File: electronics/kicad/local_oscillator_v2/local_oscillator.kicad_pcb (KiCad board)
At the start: 2 copper layers, 12 parts, among them P1 TestPoint:TestPoint_Pad_1.5x1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, P2 TestPoint:TestPoint_Pad_1.5x1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, P3 TestPoint:TestPoint_Pad_1.5x1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, U1 CE3520K3

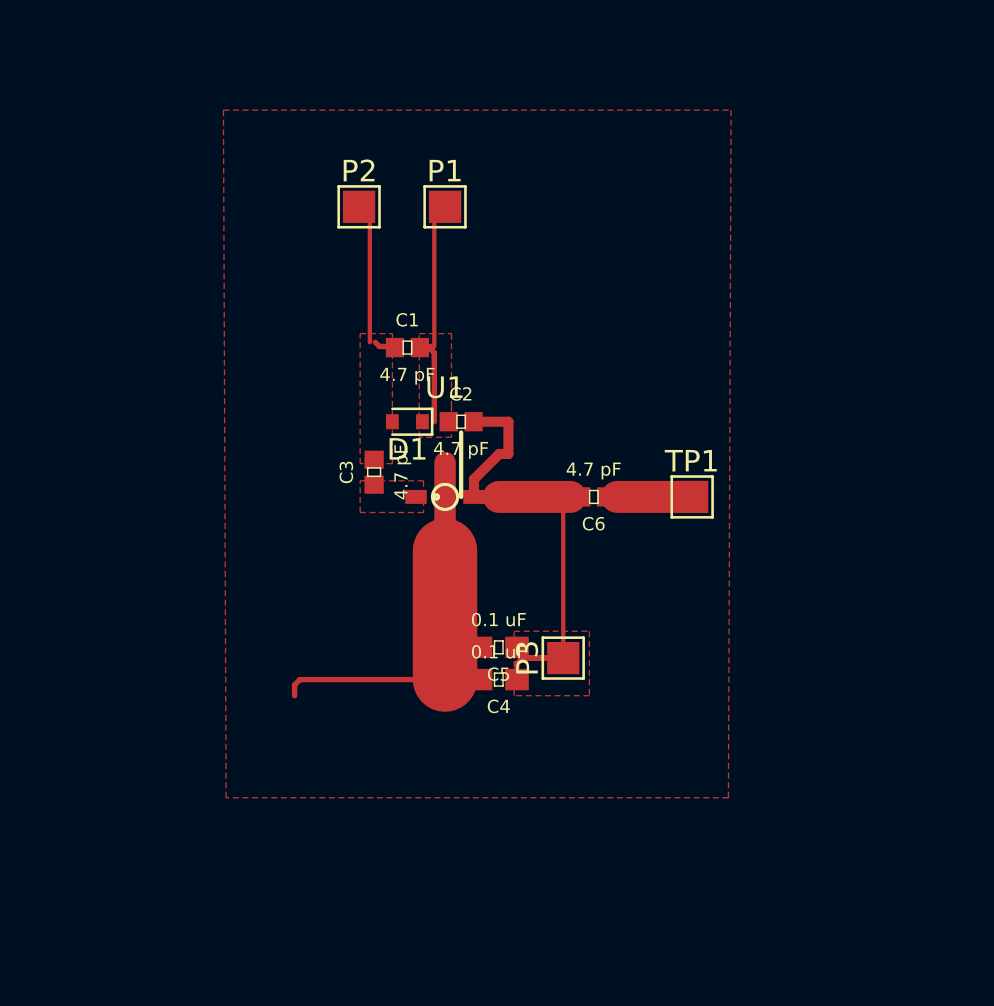
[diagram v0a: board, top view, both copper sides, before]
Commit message: Notch filter
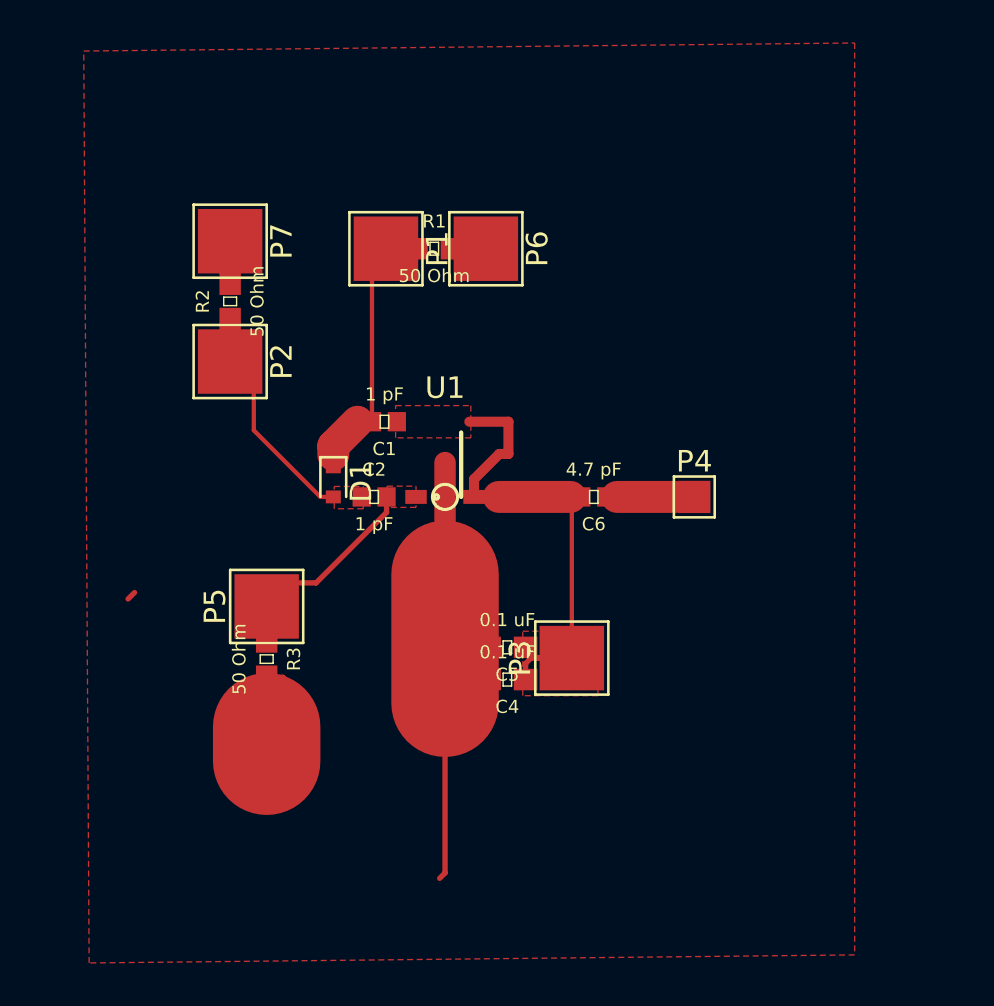
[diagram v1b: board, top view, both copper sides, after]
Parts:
- removed C3: 4.7 pF, 0402
- removed TP1: SMA, TestPoint:TestPoint_Pad_1.5x1.5mm
- added P4: TestPoint:TestPoint_Pad_1.5x1.5mm, TestPoint:TestPoint_Pad_1.5x1.5mm, F.Cu at (72.6, 44.0)
- added P5: TestPoint:TestPoint_Pad_1.5x1.5mm, TestPoint:TestPoint_Pad_3.0x3.0mm, F.Cu at (52.7, 49.1)
- added P6: TestPoint:TestPoint_Pad_1.5x1.5mm, TestPoint:TestPoint_Pad_3.0x3.0mm, F.Cu at (62.9, 32.5)
- added P7: TestPoint:TestPoint_Pad_1.5x1.5mm, TestPoint:TestPoint_Pad_3.0x3.0mm, F.Cu at (51.0, 32.1)
- added R1: 50 Ohm, Capacitors:0603, F.Cu at (60.5, 32.5)
- added R2: 50 Ohm, Capacitors:0603, F.Cu at (51.0, 34.9)
- added R3: 50 Ohm, Capacitors:0603, F.Cu at (52.7, 51.5)
- C1: value 4.7 pF -> 1 pF; footprint 0402 -> Capacitors:0402
- C2: value 4.7 pF -> 1 pF
- D1: value D -> D_Capacitance
- P1, P2, P3: footprint TestPoint:TestPoint_Pad_1.5x1.5mm -> TestPoint:TestPoint_Pad_3.0x3.0mm
- moved P2 9.37 mm to (51.0, 37.7), turned to 270 degrees
- moved C2 5.35 mm to (57.7, 44.0)
- moved D1 4.44 mm to (55.8, 43.3), turned to 270 degrees
- moved C1 3.61 mm to (58.2, 40.5), turned to 180 degrees
- moved P1 3.37 mm to (58.2, 32.5), turned to 270 degrees
- moved C4 0.40 mm to (63.9, 52.5)
- moved C5 0.40 mm to (63.9, 51.0)
- moved P3 0.40 mm to (66.9, 51.5)
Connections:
- C1 pad 1: /VCO1 -> /VCC
- C1 pad 2: /VCO2 -> Net-(C1-Pad2)
- C2 pad 1: /VCO2 -> Net-(C2-Pad1)
- C2 pad 2: /VCC -> Net-(C2-Pad2)
- D1 pad 1: /VCO2 -> Net-(C1-Pad2)
- D1 pad 2: /VCO1 -> Net-(C2-Pad1)
- P1 pad 1: /VCO2 -> Net-(C1-Pad2)
- P2 pad 1: /VCO1 -> Net-(C2-Pad1)
- U1 pad 4: /GATE -> Net-(C2-Pad2)
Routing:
- net Net-(C1-Pad2): track 0.00 -> 12.6 mm
- net /VCO2: track 10.3 -> 0.00 mm
- net /VCO1: track 6.76 -> 0.00 mm
- net Net-(C2-Pad1): track 0.00 -> 6.68 mm
- net Net-(C2-Pad2): track 0.00 -> 6.11 mm
- net GND: track 16.3 -> 21.8 mm
- net Net-(C6-Pad1): track 0.00 -> 2.75 mm
- net (no net): track 2.75 -> 0.00 mm
- added copper zone on F.Cu, net Net-(C2-Pad1)
- added copper zone on F.Cu, net Net-(C2-Pad2)
- removed copper zone on F.Cu, net /GATE
- removed copper zone on F.Cu, net /VCO1
- removed copper zone on F.Cu, net /VCO2

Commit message: aaaaaaaaaaaa
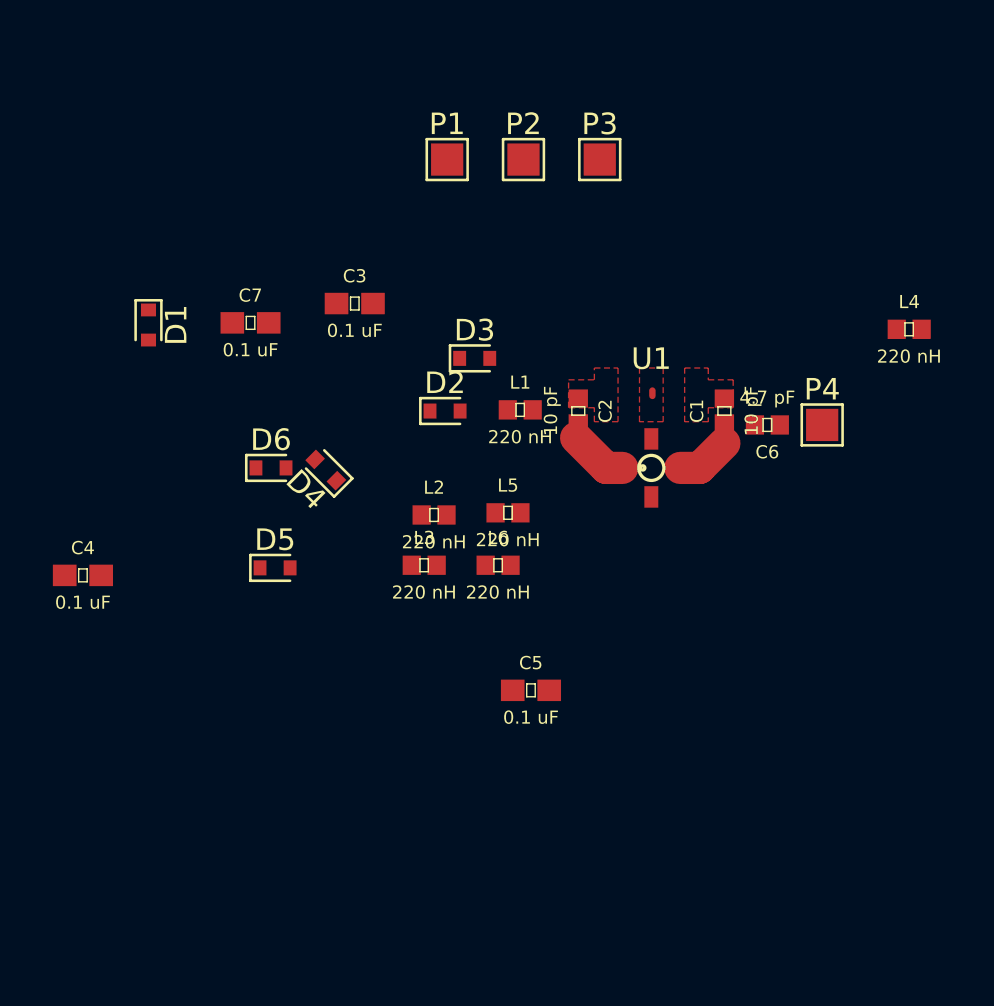
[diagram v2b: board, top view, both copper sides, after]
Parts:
- removed P5, P6, P7: TestPoint:TestPoint_Pad_1.5x1.5mm, TestPoint:TestPoint_Pad_3.0x3.0mm
- removed R1, R2, R3: 50 Ohm, Capacitors:0603
- added C3: 0.1 uF, Capacitors:0603, F.Cu at (56.8, 35.0)
- added C7: 0.1 uF, Capacitors:0603, F.Cu at (51.9, 35.9)
- added D2: D_Capacitance, Diode_SMD:D_SOD-523, F.Cu at (61.0, 40.0)
- added D3: D_Capacitance, Diode_SMD:D_SOD-523, F.Cu at (62.4, 37.6)
- added D4: D_Capacitance, Diode_SMD:D_SOD-523, F.Cu at (55.5, 42.8)
- added D5: D_Capacitance, Diode_SMD:D_SOD-523, F.Cu at (53.1, 47.3)
- added D6: D_Capacitance, Diode_SMD:D_SOD-523, F.Cu at (52.9, 42.6)
- added L1: 220 nH, Capacitors:0402, F.Cu at (64.5, 40.0)
- added L2: 220 nH, Capacitors:0402, F.Cu at (60.5, 44.8)
- added L3: 220 nH, Capacitors:0402, F.Cu at (60.0, 47.2)
- added L4: 220 nH, Capacitors:0402, F.Cu at (82.6, 36.2)
- added L5: 220 nH, Capacitors:0402, F.Cu at (63.9, 44.7)
- added L6: 220 nH, Capacitors:0402, F.Cu at (63.5, 47.2)
- C1, C2: value 1 pF -> 10 pF
- P1, P2, P3: footprint TestPoint:TestPoint_Pad_3.0x3.0mm -> TestPoint:TestPoint_Pad_1.5x1.5mm
- moved P3 23.2 mm to (68.2, 28.3), turned to 0 degrees
- moved C4 20.3 mm to (44.1, 47.7), turned to 0 degrees
- moved P2 16.6 mm to (64.7, 28.3), turned to 0 degrees
- moved C1 15.8 mm to (74.0, 40.0), turned to 90 degrees
- moved D1 11.3 mm to (47.2, 36.0)
- moved C2 10.3 mm to (67.2, 40.0), turned to 270 degrees
- moved U1 9.69 mm to (70.6, 42.6)
- moved C6 8.75 mm to (76.0, 40.6)
- moved P4 6.83 mm to (78.5, 40.6)
- moved P1 5.03 mm to (61.1, 28.3), turned to 0 degrees
- moved C5 2.28 mm to (65.0, 53.0), turned to 0 degrees
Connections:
- C1 pad 2: Net-(C1-Pad2) -> GND
- C2 pad 1: Net-(C2-Pad1) -> GND
- D1 pad 1: Net-(C1-Pad2) -> GND
- D1 pad 2: Net-(C2-Pad1) -> Net-(D1-Pad2)
- P1 pad 1: Net-(C1-Pad2) -> Net-(C3-Pad2)
- P2 pad 1: Net-(C2-Pad1) -> Net-(C7-Pad1)
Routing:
- net GND: track 21.8 -> 0.00 mm
- net /VCC: track 22.3 -> 2.53 mm
- net Net-(C1-Pad2): track 12.6 -> 0.00 mm
- net Net-(C2-Pad1): track 6.68 -> 0.00 mm
- net Net-(C2-Pad2): track 6.11 -> 2.73 mm
- net Net-(C6-Pad1): track 2.75 -> 0.00 mm
- added copper zone on F.Cu, net /FLT
- removed copper zone on F.Cu, net /VCC
- removed copper zone on F.Cu, net Net-(C2-Pad1)
- removed copper zone on F.Cu, net Net-(C2-Pad2)
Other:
- net class Default: trace_width 0.25 -> 1.5

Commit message: goddamnit
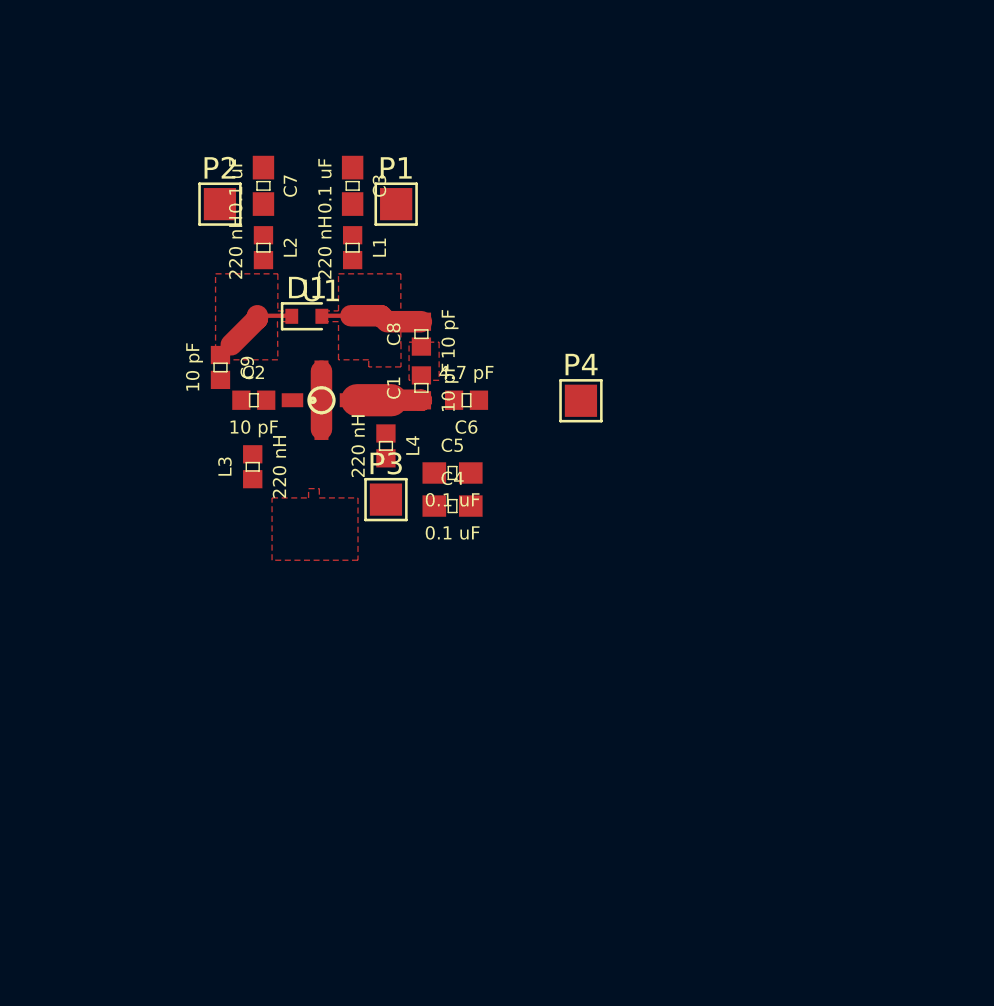
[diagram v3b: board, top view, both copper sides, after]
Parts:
- removed D2, D3, D4, D5, D6: D_Capacitance, Diode_SMD:D_SOD-523
- removed L5, L6: 220 nH, Capacitors:0402
- added C8: 10 pF, Capacitors:0402, F.Cu at (59.9, 36.4)
- added C9: 10 pF, Capacitors:0402, F.Cu at (50.5, 38.0)
- moved L4 24.9 mm to (58.2, 41.6), turned to 270 degrees
- moved P3 18.7 mm to (58.2, 44.1)
- moved C4 17.5 mm to (61.4, 44.4)
- moved U1 15.7 mm to (55.2, 39.5)
- moved C2 15.1 mm to (52.1, 39.5), turned to 0 degrees
- moved L2 14.8 mm to (52.5, 32.4), turned to 270 degrees
- moved P2 14.3 mm to (50.5, 30.4)
- moved C1 14.1 mm to (59.9, 38.9)
- moved C6 14.0 mm to (62.0, 39.5)
- moved P4 11.3 mm to (67.3, 39.5)
- moved L1 10.9 mm to (56.7, 32.4), turned to 270 degrees
- moved C5 10.8 mm to (61.3, 42.9)
- moved L3 9.20 mm to (52.0, 42.6), turned to 90 degrees
- moved D1 7.38 mm to (54.6, 35.6), turned to 0 degrees
- moved C7 6.40 mm to (52.5, 29.5), turned to 270 degrees
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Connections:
- C1 pad 2: GND -> Net-(C1-Pad2)
- C2 pad 1: GND -> Net-(C2-Pad1)
- C4 pad 1: /VCC -> Net-(C4-Pad1)
- C5 pad 1: /VCC -> Net-(C4-Pad1)
- C7 pad 1: Net-(C7-Pad1) -> GND
- C7 pad 2: GND -> Net-(C7-Pad2)
- D1 pad 1: GND -> /FLT1
- D1 pad 2: Net-(D1-Pad2) -> /FLT2
- L1 pad 1: GND -> Net-(C3-Pad2)
- L1 pad 2: Net-(C3-Pad2) -> /FLT2
- L2 pad 1: Net-(D1-Pad2) -> Net-(C7-Pad2)
- L2 pad 2: Net-(C7-Pad1) -> /FLT1
- L3 pad 2: GND -> Net-(C2-Pad2)
- L4 pad 1: Net-(D3-Pad2) -> /VCC
- L4 pad 2: Net-(D1-Pad2) -> Net-(C4-Pad1)
- P2 pad 1: Net-(C7-Pad1) -> Net-(C7-Pad2)
- P3 pad 1: /VCC -> Net-(C4-Pad1)
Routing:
- net /FLT2: track 0.00 -> 4.60 mm
- net /FLT1: track 0.00 -> 3.51 mm
- net Net-(C2-Pad2): track 2.73 -> 0.00 mm
- net GND: track 0.00 -> 2.70 mm
- added copper zone on F.Cu, net (none)
- added copper zone on F.Cu, net /FLT1
- added copper zone on F.Cu, net /FLT2
- added copper zone on F.Cu, net Net-(C1-Pad2)
- removed copper zone on F.Cu, net /FLT
- removed copper zone on F.Cu, net GND
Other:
- net class Default: trace_width 1.5 -> 1
- net class b added: clearance 0.2, trace_width 0.2, via_dia 0.8, via_drill 0.4
